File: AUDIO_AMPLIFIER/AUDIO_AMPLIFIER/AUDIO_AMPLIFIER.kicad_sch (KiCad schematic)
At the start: 13 parts, among them J1 Screw_Terminal_01x02, J2 Screw_Terminal_01x02, U1 LM386

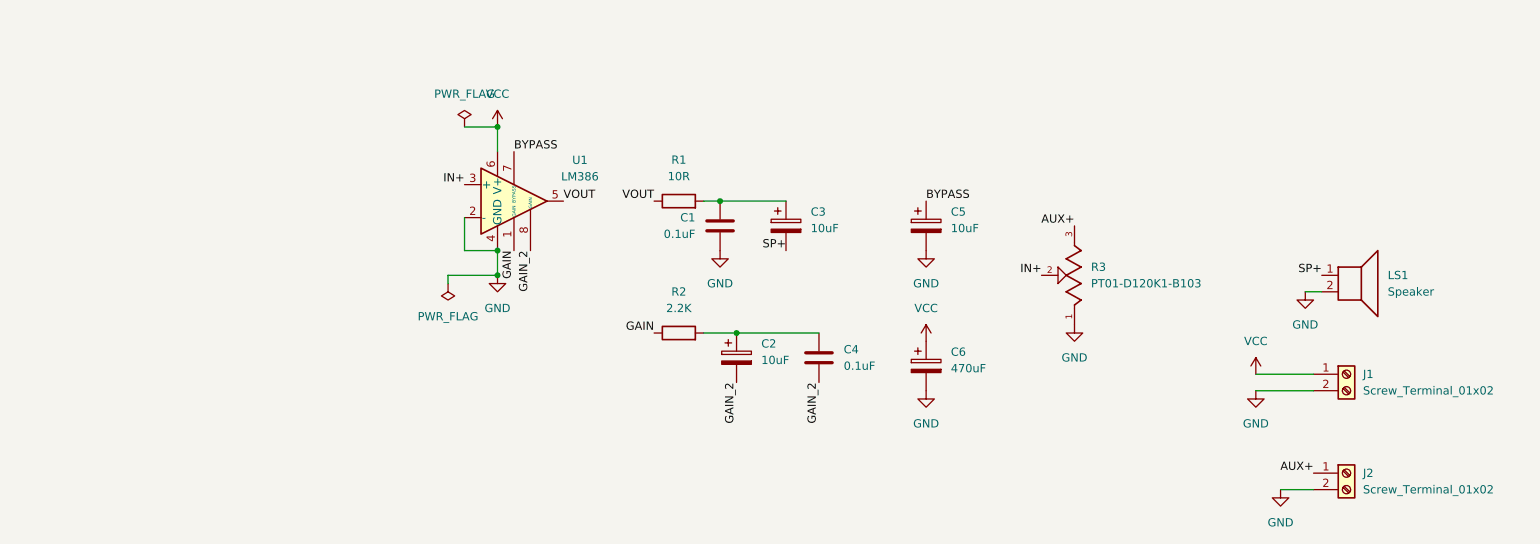
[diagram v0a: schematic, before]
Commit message: BMS made
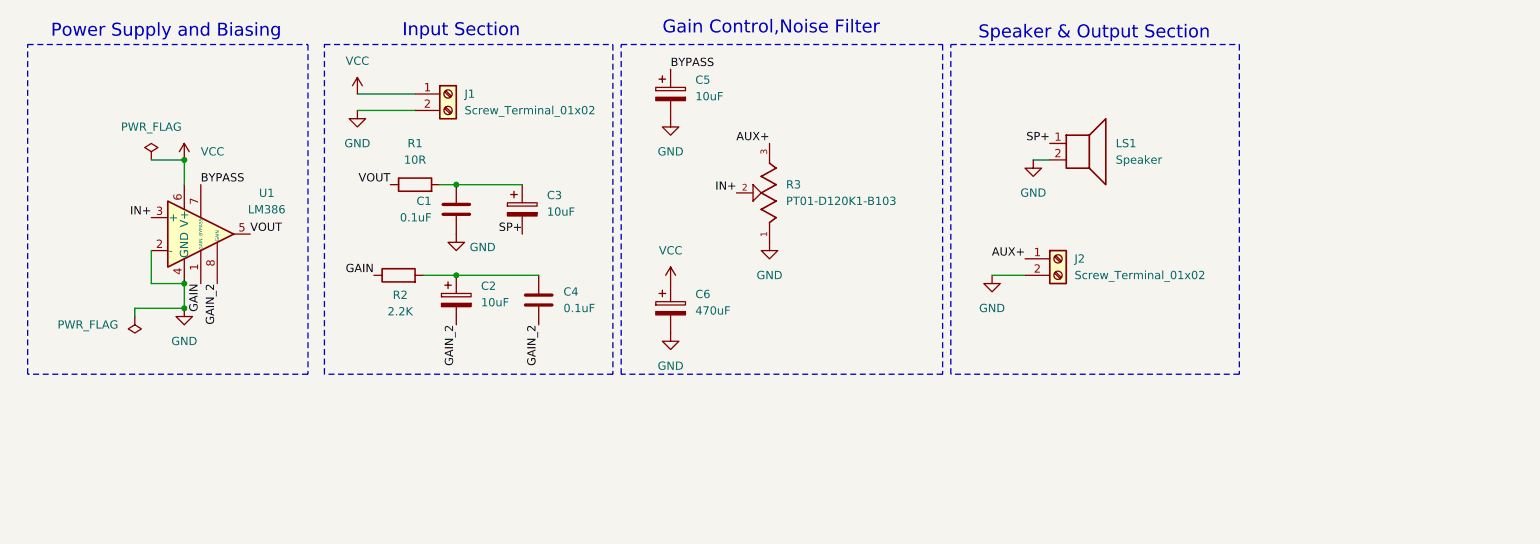
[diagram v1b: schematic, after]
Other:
- note added: "Gain Control,Noise Filter"
- note added: "Input Section"
- note added: "Power Supply and Biasing"
- note added: "Speaker & Output Section"
- title: (none) -> AUDIO_AMPLIFIER
- moved on the sheet: C1, C2, C3, C4, C5, C6, J1, J2, LS1, R1, R2, R3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
